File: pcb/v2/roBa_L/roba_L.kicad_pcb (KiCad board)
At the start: 2 copper layers, 123.9 x 94.5 mm, 56 parts, among them J1 Conn_01x01-Connector_Generic, J2 Conn_01x01-Connector_Generic, J3 Conn_01x01-Connector_Generic, J4 Conn_01x01-Connector_Generic, J5 Conn_01x01-Connector_Generic, J6 Conn_01x01-Connector_Generic, J7 Conn_01x01-Connector_Generic, SW1 SW_PUSH, SW10 SW_PUSH, SW11 SW_PUSH, SW12 SW_PUSH, SW13 SW_PUSH, SW14 SW_PUSH, SW15 SW_PUSH, SW16 SW_PUSH, SW17 SW_PUSH, SW18 SW_PUSH, SW19 SW_PUSH, SW2 SW_PUSH, SW20 SW_PUSH, SW21 RotaryEncoder_Switch, SW22 SW_PUSH, SW23 SW_PUSH, SW24 SW_SPDT, SW3 SW_PUSH, SW4 SW_PUSH, SW5 SW_PUSH, SW6 SW_PUSH, SW7 SW_PUSH, SW8 SW_PUSH, SW9 SW_PUSH

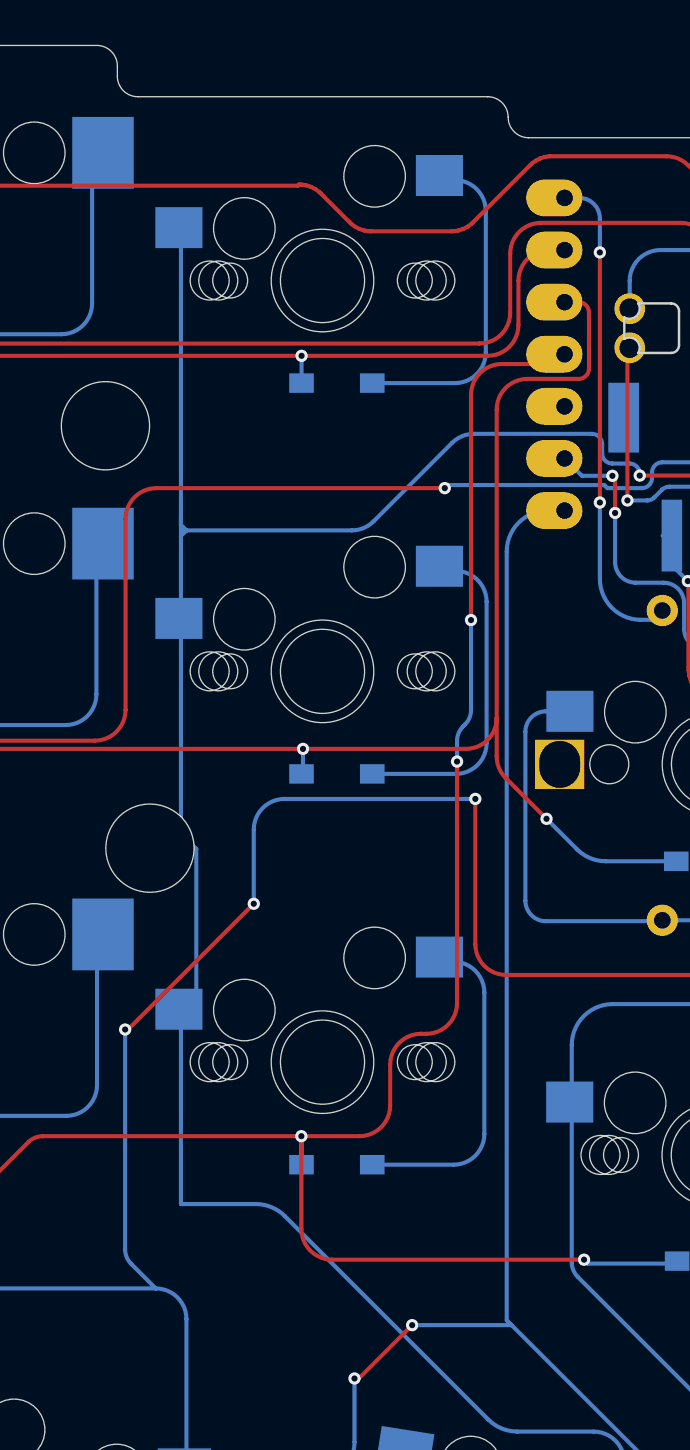
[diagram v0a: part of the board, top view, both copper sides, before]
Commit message: Lの五列目ok
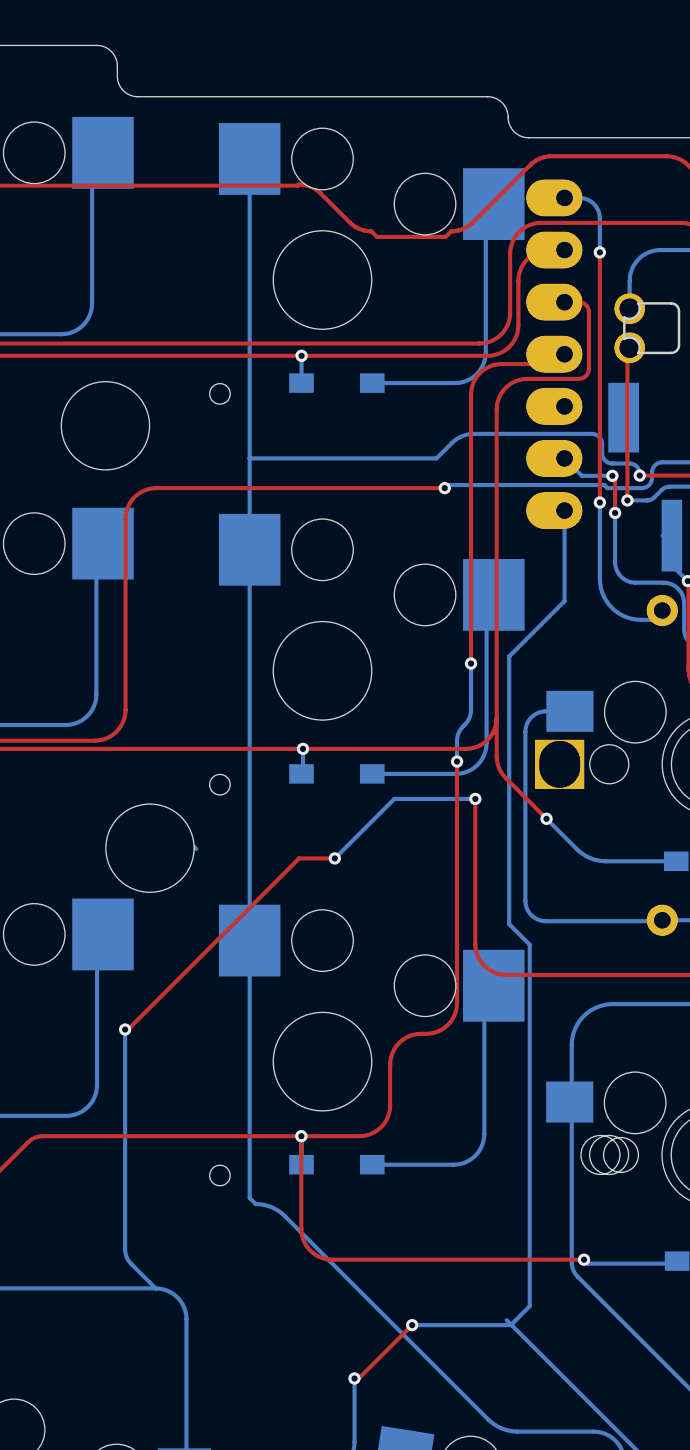
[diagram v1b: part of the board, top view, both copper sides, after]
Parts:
- SW17, SW18, SW19: footprint roBa:SW_MX -> ChocV2_Hotswap:Choc_v2_Hotswap_1u_MXcompatible.pretty
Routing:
- net Col4: track 126.1 -> 120.6 mm
- net Net-(D18-A): track 16.3 -> 13.3 mm
- net Net-(D17-A): track 16.2 -> 13.2 mm
- net Net-(D19-A): track 16.0 -> 13.2 mm
- net Col3: track 176.3 -> 174.0 mm
- net Row3: track 204.4 -> 205.4 mm

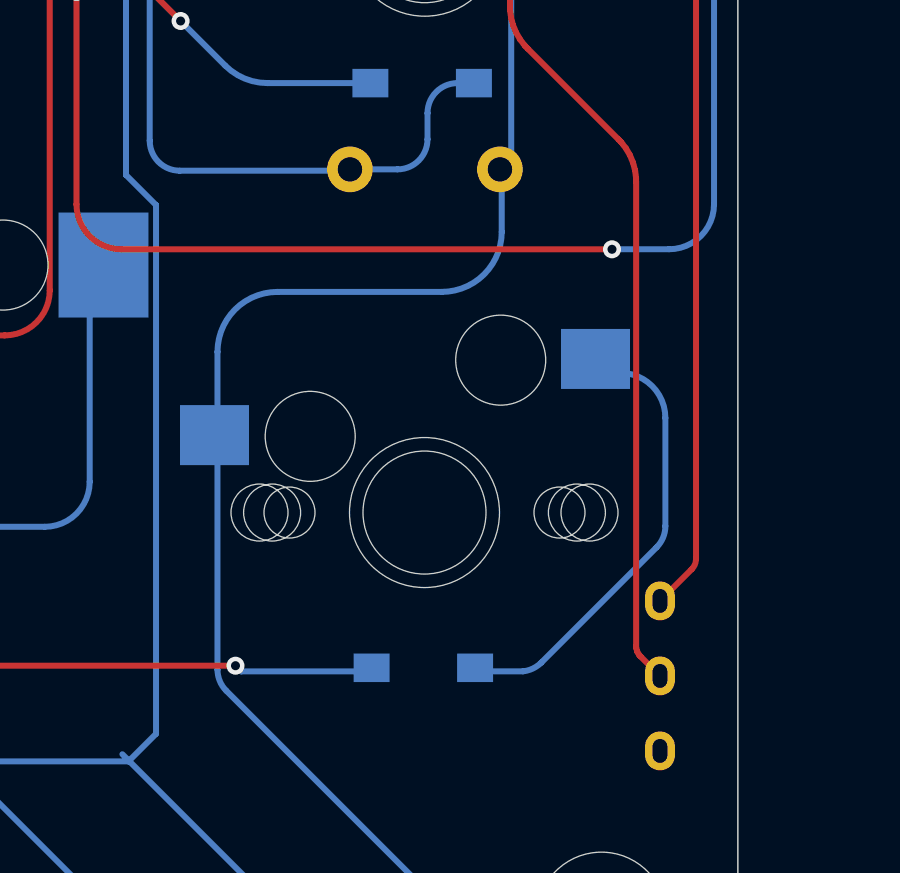
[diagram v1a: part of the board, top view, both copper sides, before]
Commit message: 出力前
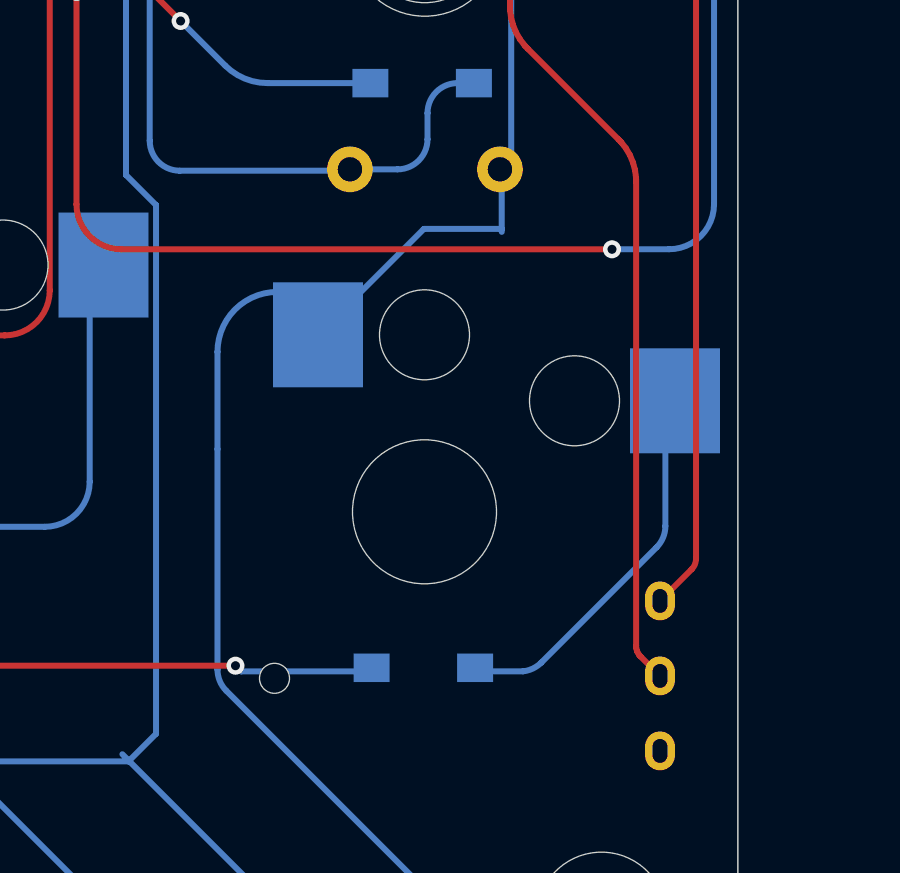
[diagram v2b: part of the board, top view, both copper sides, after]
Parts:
- SW22: footprint roBa:SW_MX -> ChocV2_Hotswap:Choc_v2_Hotswap_1u_MXcompatible.pretty
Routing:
- net Net-(D22-A): track 15.2 -> 12.2 mm
- net Col5: track 85.6 -> 84.7 mm
